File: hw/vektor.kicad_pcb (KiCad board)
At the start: 6 copper layers, 100 x 44 mm, 259 parts, among them J1 Header_2.54mm_10p, J2 0430450818, M1 MHNP_2.5mm, M2 MHNP_2.5mm, M3 MHNP_2.5mm, M4 MHNP_2.5mm, M5 MHNP_2.5mm, Q1 PHPT61002PYCLHX, Q2 PUMH13, Q3 PUMD13, U1 TAS2770, U10 74LVCH1T45GW, U11 74LVCH1T45GW, U12 74LVCH1T45GW, U13 74LVCH1T45GW, U14 74LVCH1T45GW, U15 74LVCH1T45GW, U16 LMZ10501SILR, U17 LMZ10501SILR, U2 TAS2770, U3 TAS2770, U4 ADAU1467, U5 TORX1355(V,F), U6 TOTX1350(V,F), U7 25AA1024, U8 LP3470IM5X-3.08_NOPB, U9 XCL226A0K1H2, X1 NX3225SA-12.288M-STD-CRS-2

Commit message: ...
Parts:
- U5, U6: footprint TOSLINK_VERTICAL -> footprints:TOSLINK_VERTICAL
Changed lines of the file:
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@@
-(kicad_pcb (version 20171130) (host pcbnew "(5.1.0-0)")
+(kicad_pcb (version 20171130) (host pcbnew "(5.1.2-1)-1")
   (general
     (thickness 1.6)
@@
     (add_net P5V0)
   )
+  (module footprints:TOSLINK_VERTICAL (layer B.Cu)
+    (at 141 85 90)
+    (fp_text reference U5 (at 0 -1.905 90) (layer B.SilkS)
+      (effects (font (size 0.8 0.8) (thickness 0.127)) (justify mirror))
+    )
+    (fp_text value "TORX1355(V,F)" (at 0 -6.35 90) (layer B.Fab)
+      (effects (font (size 1 1) (thickness 0.15)) (justify mirror))
+    )
+    (fp_text user TOSLINK (at 0 4.445 90) (layer B.SilkS)
+      (effects (font (size 1 1) (thickness 0.15)) (justify mirror))
+    )
+    (fp_circle (center 0 0.635) (end 0 1.905) (layer B.SilkS) (width 0.15))
+    (fp_line (start 2.54 -2.54) (end -2.54 -2.54) (layer B.SilkS) (width 0.15))
+    (fp_line (start 3.81 -1.27) (end 2.54 -2.54) (layer B.SilkS) (width 0.15))
+    (fp_line (start 3.81 3.81) (end 3.81 -1.27) (layer B.SilkS) (width 0.15))
+    (fp_line (start -3.81 3.81) (end 3.81 3.81) (layer B.SilkS) (width 0.15))
+    (fp_line (start -3.81 -1.27) (end -3.81 3.81) (layer B.SilkS) (width 0.15))
+    (fp_line (start -2.54 -2.54) (end -3.81 -1.27) (layer B.SilkS) (width 0.15))
+    (fp_line (start -7.7 5.25) (end -7.7 -5.25) (layer B.SilkS) (width 0.15))
+    (fp_line (start 7.7 5.25) (end 7.7 -5.25) (layer B.SilkS) (width 0.15))
+    (fp_line (start -7.7 -5.25) (end 7.7 -5.25) (layer B.SilkS) (width 0.15))
+    (fp_line (start -7.7 5.25) (end 7.7 5.25) (layer B.SilkS) (width 0.15))
+    (pad 5 thru_hole circle (at 6.525 0 90) (size 1.524 1.524) (drill 0.762) (layers *.Cu *.Mask)
+      (net 41 "Net-(U5-Pad5)"))
+    (pad 4 thru_hole circle (at -6.525 0 90) (size 1.524 1.524) (drill 0.762) (layers *.Cu *.Mask)
+      (net 40 "Net-(U5-Pad4)"))
+    (pad 3 thru_hole circle (at -2.54 -3.85 90) (size 1.524 1.524) (drill 0.762) (layers *.Cu *.Mask)
+      (net 113 P5V0))
+    (pad 2 thru_hole circle (at 0 -3.85 90) (size 1.524 1.524) (drill 0.762) (layers *.Cu *.Mask)
+      (net 1 GND))
+    (pad 1 thru_hole circle (at 2.54 -3.85 90) (size 1.524 1.524) (drill 0.762) (layers *.Cu *.Mask)
+      (net 132 "Net-(TP57-Pad1)"))
+    (model toslink.step
+      (at (xyz 0 0 0))
+      (scale (xyz 1 1 1))
+      (rotate (xyz 0 0 0))
+    )
+  )
+  (module footprints:TOSLINK_VERTICAL (layer B.Cu)
+    (at 141 111 90)
+    (fp_text reference U6 (at 0 -1.905 90) (layer B.SilkS)
+      (effects (font (size 0.8 0.8) (thickness 0.127)) (justify mirror))
+    )
+    (fp_text value "TOTX1350(V,F)" (at 0 -6.35 90) (layer B.Fab)
+      (effects (font (size 1 1) (thickness 0.15)) (justify mirror))
+    )
+    (fp_text user TOSLINK (at 0 4.445 90) (layer B.SilkS)
+      (effects (font (size 1 1) (thickness 0.15)) (justify mirror))
+    )
+    (fp_circle (center 0 0.635) (end 0 1.905) (layer B.SilkS) (width 0.15))
+    (fp_line (start 2.54 -2.54) (end -2.54 -2.54) (layer B.SilkS) (width 0.15))
+    (fp_line (start 3.81 -1.27) (end 2.54 -2.54) (layer B.SilkS) (width 0.15))
+    (fp_line (start 3.81 3.81) (end 3.81 -1.27) (layer B.SilkS) (width 0.15))
+    (fp_line (start -3.81 3.81) (end 3.81 3.81) (layer B.SilkS) (width 0.15))
+    (fp_line (start -3.81 -1.27) (end -3.81 3.81) (layer B.SilkS) (width 0.15))
+    (fp_line (start -2.54 -2.54) (end -3.81 -1.27) (layer B.SilkS) (width 0.15))
+    (fp_line (start -7.7 5.25) (end -7.7 -5.25) (layer B.SilkS) (width 0.15))
+    (fp_line (start 7.7 5.25) (end 7.7 -5.25) (layer B.SilkS) (width 0.15))
+    (fp_line (start -7.7 -5.25) (end 7.7 -5.25) (layer B.SilkS) (width 0.15))
+    (fp_line (start -7.7 5.25) (end 7.7 5.25) (layer B.SilkS) (width 0.15))
+    (pad 5 thru_hole circle (at 6.525 0 90) (size 1.524 1.524) (drill 0.762) (layers *.Cu *.Mask)
+      (net 42 "Net-(U6-Pad5)"))
+    (pad 4 thru_hole circle (at -6.525 0 90) (size 1.524 1.524) (drill 0.762) (layers *.Cu *.Mask)
+      (net 43 "Net-(U6-Pad4)"))
+    (pad 3 thru_hole circle (at -2.54 -3.85 90) (size 1.524 1.524) (drill 0.762) (layers *.Cu *.Mask)
+      (net 128 "Net-(R19-Pad2)"))
+    (pad 2 thru_hole circle (at 0 -3.85 90) (size 1.524 1.524) (drill 0.762) (layers *.Cu *.Mask)
+      (net 1 GND))
+    (pad 1 thru_hole circle (at 2.54 -3.85 90) (size 1.524 1.524) (drill 0.762) (layers *.Cu *.Mask)
+      (net 44 "Net-(U6-Pad1)"))
+    (model toslink.step
+      (at (xyz 0 0 0))
+      (scale (xyz 1 1 1))
+      (rotate (xyz 0 0 0))
+    )
+  )
   (module footprints:TP_1mm (layer F.Cu)
     (at 202.3 92.3)
@@
     )
   )
-  (module TOSLINK_VERTICAL (layer B.Cu)
-    (at 141 85 90)
-    (fp_text reference U5 (at 0 -1.905 90) (layer B.SilkS)
-      (effects (font (size 0.8 0.8) (thickness 0.127)) (justify mirror))
-    )
-    (fp_text value "TORX1355(V,F)" (at 0 -6.35 90) (layer B.Fab)
-      (effects (font (size 1 1) (thickness 0.15)) (justify mirror))
-    )
-    (fp_line (start -7.7 5.25) (end 7.7 5.25) (layer B.SilkS) (width 0.15))
-    (fp_line (start -7.7 -5.25) (end 7.7 -5.25) (layer B.SilkS) (width 0.15))
-    (fp_line (start 7.7 5.25) (end 7.7 -5.25) (layer B.SilkS) (width 0.15))
-    (fp_line (start -7.7 5.25) (end -7.7 -5.25) (layer B.SilkS) (width 0.15))
-    (fp_line (start -2.54 -2.54) (end -3.81 -1.27) (layer B.SilkS) (width 0.15))
-    (fp_line (start -3.81 -1.27) (end -3.81 3.81) (layer B.SilkS) (width 0.15))
-    (fp_line (start -3.81 3.81) (end 3.81 3.81) (layer B.SilkS) (width 0.15))
-    (fp_line (start 3.81 3.81) (end 3.81 -1.27) (layer B.SilkS) (width 0.15))
-    (fp_line (start 3.81 -1.27) (end 2.54 -2.54) (layer B.SilkS) (width 0.15))
-    (fp_line (start 2.54 -2.54) (end -2.54 -2.54) (layer B.SilkS) (width 0.15))
-    (fp_circle (center 0 0.635) (end 0 1.905) (layer B.SilkS) (width 0.15))
-    (fp_text user TOSLINK (at 0 4.445 90) (layer B.SilkS)
-      (effects (font (size 1 1) (thickness 0.15)) (justify mirror))
-    )
-    (pad 1 thru_hole circle (at 2.54 -3.85 90) (size 1.524 1.524) (drill 0.762) (layers *.Cu *.Mask)
-      (net 132 "Net-(TP57-Pad1)"))
-    (pad 2 thru_hole circle (at 0 -3.85 90) (size 1.524 1.524) (drill 0.762) (layers *.Cu *.Mask)
-      (net 1 GND))
-    (pad 3 thru_hole circle (at -2.54 -3.85 90) (size 1.524 1.524) (drill 0.762) (layers *.Cu *.Mask)
-      (net 113 P5V0))
-    (pad 4 thru_hole circle (at -6.525 0 90) (size 1.524 1.524) (drill 0.762) (layers *.Cu *.Mask)
-      (net 40 "Net-(U5-Pad4)"))
-    (pad 5 thru_hole circle (at 6.525 0 90) (size 1.524 1.524) (drill 0.762) (layers *.Cu *.Mask)
-      (net 41 "Net-(U5-Pad5)"))
-  )
-  (module TOSLINK_VERTICAL (layer B.Cu)
-    (at 141 111 90)
-    (fp_text reference U6 (at 0 -1.905 90) (layer B.SilkS)
-      (effects (font (size 0.8 0.8) (thickness 0.127)) (justify mirror))
-    )
-    (fp_text value "TOTX1350(V,F)" (at 0 -6.35 90) (layer B.Fab)
-      (effects (font (size 1 1) (thickness 0.15)) (justify mirror))
-    )
-    (fp_text user TOSLINK (at 0 4.445 90) (layer B.SilkS)
-      (effects (font (size 1 1) (thickness 0.15)) (justify mirror))
-    )
-    (fp_circle (center 0 0.635) (end 0 1.905) (layer B.SilkS) (width 0.15))
-    (fp_line (start 2.54 -2.54) (end -2.54 -2.54) (layer B.SilkS) (width 0.15))
-    (fp_line (start 3.81 -1.27) (end 2.54 -2.54) (layer B.SilkS) (width 0.15))
-    (fp_line (start 3.81 3.81) (end 3.81 -1.27) (layer B.SilkS) (width 0.15))
-    (fp_line (start -3.81 3.81) (end 3.81 3.81) (layer B.SilkS) (width 0.15))
-    (fp_line (start -3.81 -1.27) (end -3.81 3.81) (layer B.SilkS) (width 0.15))
-    (fp_line (start -2.54 -2.54) (end -3.81 -1.27) (layer B.SilkS) (width 0.15))
-    (fp_line (start -7.7 5.25) (end -7.7 -5.25) (layer B.SilkS) (width 0.15))
-    (fp_line (start 7.7 5.25) (end 7.7 -5.25) (layer B.SilkS) (width 0.15))
-    (fp_line (start -7.7 -5.25) (end 7.7 -5.25) (layer B.SilkS) (width 0.15))
-    (fp_line (start -7.7 5.25) (end 7.7 5.25) (layer B.SilkS) (width 0.15))
-    (pad 5 thru_hole circle (at 6.525 0 90) (size 1.524 1.524) (drill 0.762) (layers *.Cu *.Mask)
-      (net 42 "Net-(U6-Pad5)"))
-    (pad 4 thru_hole circle (at -6.525 0 90) (size 1.524 1.524) (drill 0.762) (layers *.Cu *.Mask)
-      (net 43 "Net-(U6-Pad4)"))
-    (pad 3 thru_hole circle (at -2.54 -3.85 90) (size 1.524 1.524) (drill 0.762) (layers *.Cu *.Mask)
-      (net 128 "Net-(R19-Pad2)"))
-    (pad 2 thru_hole circle (at 0 -3.85 90) (size 1.524 1.524) (drill 0.762) (layers *.Cu *.Mask)
-      (net 1 GND))
-    (pad 1 thru_hole circle (at 2.54 -3.85 90) (size 1.524 1.524) (drill 0.762) (layers *.Cu *.Mask)
-      (net 44 "Net-(U6-Pad1)"))
-  )
   (module RJQ0026A (layer F.Cu)

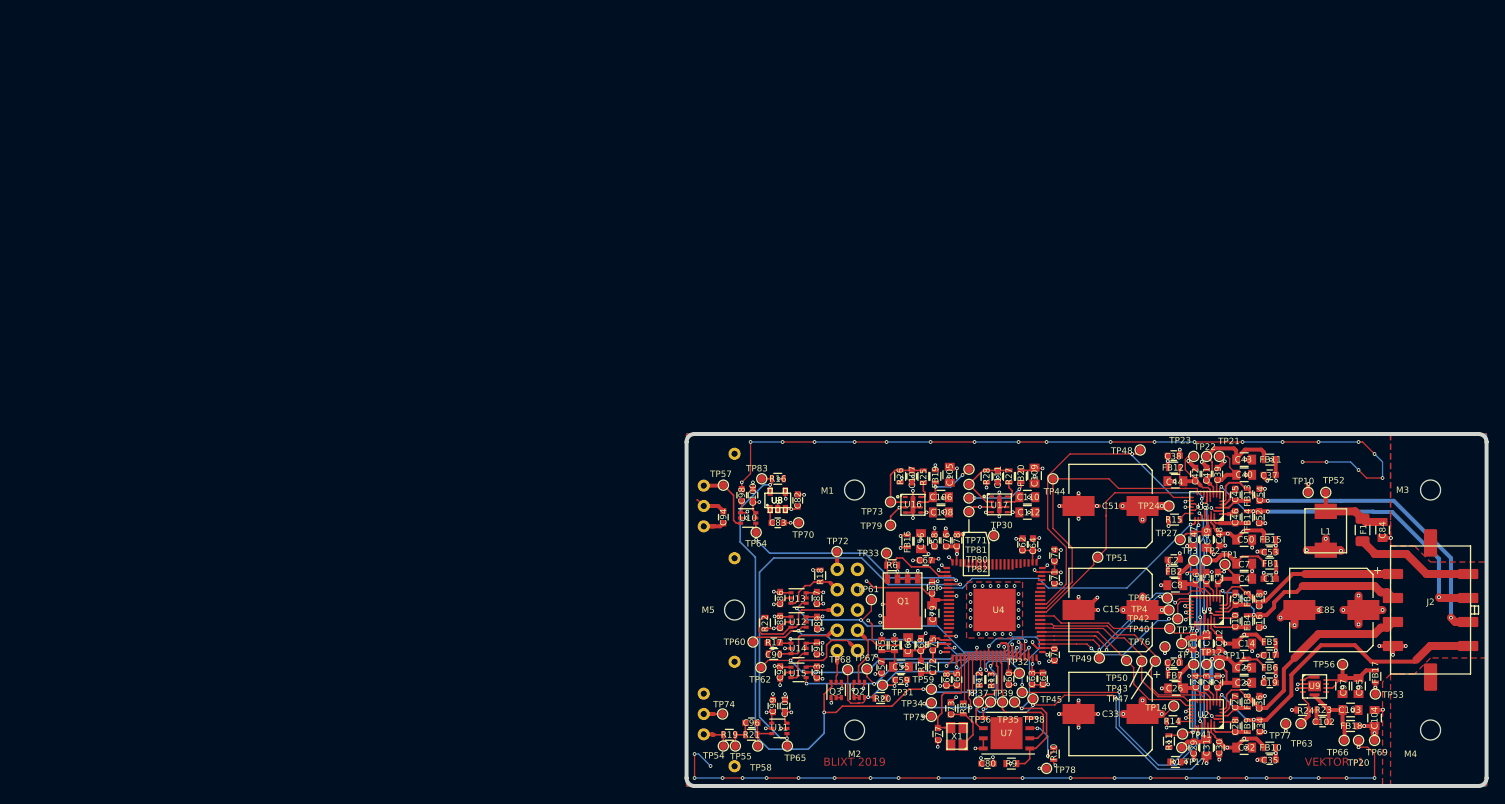
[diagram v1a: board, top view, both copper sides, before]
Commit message: preparing r2
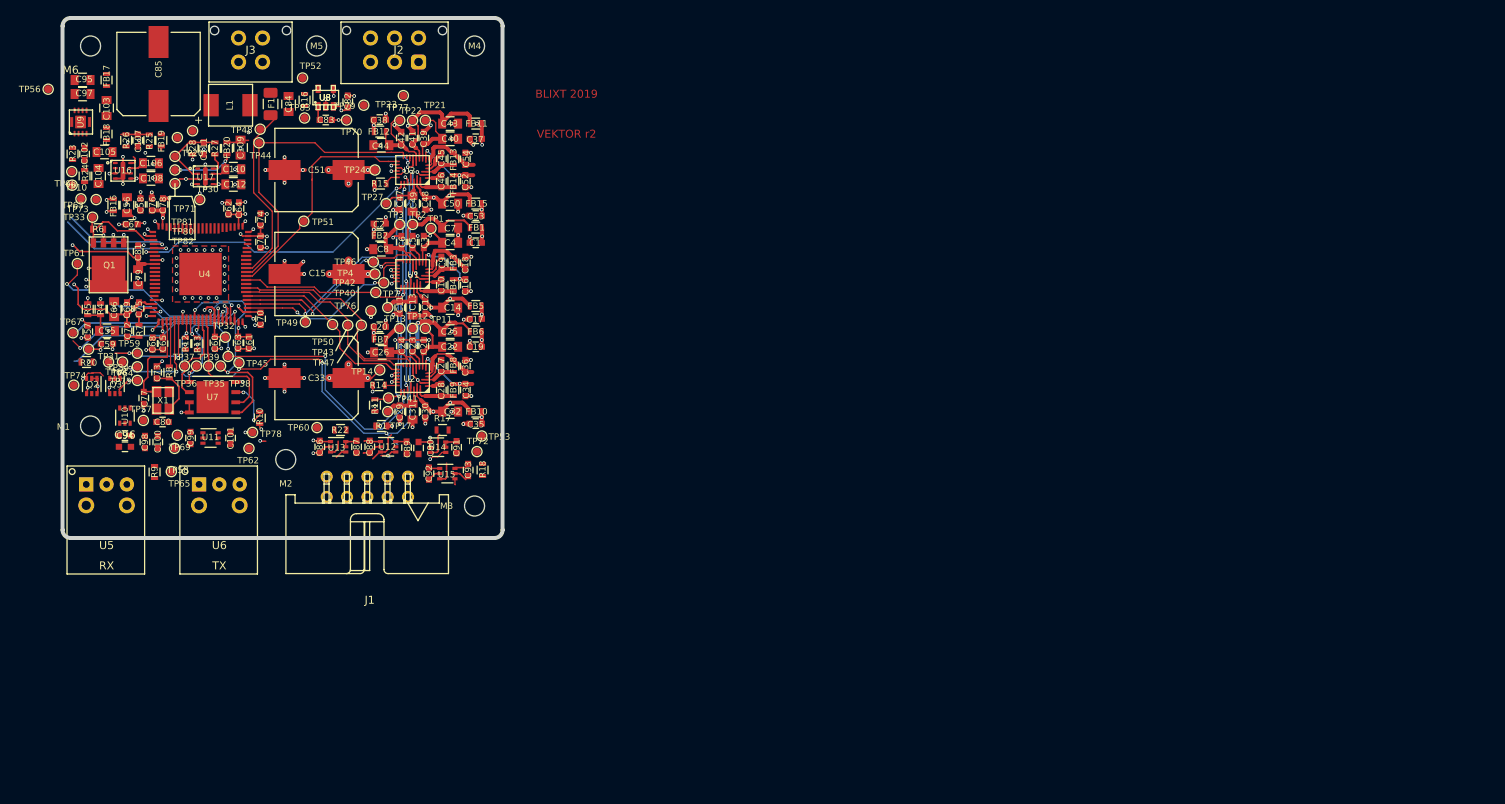
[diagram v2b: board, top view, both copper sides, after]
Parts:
- removed R19: R0603_120R, R0603
- removed R21: R0603_390R, R0603
- removed TP54, TP55: TP, footprints:TP_1mm
- added J3: 430450427, Molex_430450427, F.Cu at (80.5, 28.0)
- added M6: MHNP_2.5mm, footprints:MH_2.5mm, F.Cu at (60.5, 27.5)
- C102: value C0603_18p_50Vdc_C0G_2 -> C0603_18p_100Vdc_C0G
- C107, C111: value C0603_470p_50Vdc_C0G_2 -> C0603_470p_100Vdc_C0G
- C16, C18, C34, C36, C52, C54: value C0603_1n1_50Vdc_X7R -> C0603_1n2_50Vdc_C0G
- C84, C95: value C0805_10u_25Vdc_X7R -> C0805_10u_25Vdc_X7R(Murata)
- C96: value C0603_47p_50Vdc_C0G_2 -> C0603_1u_16Vdc_X7R
- J1: value Header_2.54mm_10p -> TE_5103310-1; footprint footprints:61201021621 -> footprints:TE_5103310_1; moved to F.Cu
- J2: value 0430450818 -> 430450629; footprint Molex_0430450818 -> Molex_430450629
- U5: value TORX1355(V,F) -> PLR135_T10; footprint footprints:TOSLINK_VERTICAL -> PLR135_T10; moved to F.Cu
- U6: value TOTX1350(V,F) -> PLT133_T10W; footprint footprints:TOSLINK_VERTICAL -> PLT133_T10W; moved to F.Cu
- moved TP56 177.1 mm to (55.2, 32.9)
- moved C95 176.6 mm to (59.5, 31.8), turned to 0 degrees
- moved FB17 175.2 mm to (62.5, 31.8)
- moved TP66 174.2 mm to (58.1, 43.2)
- moved C97 174.0 mm to (59.5, 33.5), turned to 0 degrees
- moved C104 173.3 mm to (61.5, 43.8)
- moved C103 172.8 mm to (62.5, 35.2), turned to 90 degrees
- moved FB18 172.2 mm to (62.5, 38.5), turned to 270 degrees
- moved R23 171.0 mm to (58.2, 41.0), turned to 270 degrees
- moved C102 170.3 mm to (59.8, 41.0), turned to 270 degrees
- moved U9 169.6 mm to (59.2, 37.0), turned to 90 degrees
- moved TP63 167.7 mm to (58.2, 44.9)
- moved R24 166.2 mm to (59.8, 43.8), turned to 270 degrees
- moved TP20 164.5 mm to (73.2, 38.1)
- moved C85 161.2 mm to (69.0, 31.0), turned to 90 degrees
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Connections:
- C96 pad 1: Net-(C96-Pad1) -> P5V0
- C96 pad 2: Net-(C96-Pad2) -> GND
- F1 pad 1: /VIN -> Net-(F1-Pad1)
- F1 pad 2: Net-(F1-Pad2) -> /VIN
- J2 pad 1: GND -> /Amplifier 3/AMP_OUT_P_FLT
- J2 pad 5: /Amplifier 2/AMP_OUT_N_FLT -> /Amplifier 3/AMP_OUT_N_FLT
- J2 pad 6: /Amplifier 3/AMP_OUT_P_FLT -> /Amplifier 2/AMP_OUT_N_FLT
- TP58 pad 1: Net-(C96-Pad1) -> Net-(TP58-Pad1)
- U10 pad 5: P1V8 -> P5V0
- U11 pad 3: Net-(C96-Pad1) -> Net-(TP58-Pad1)
- U12 pad 5: P1V8 -> GND
- U13 pad 5: P1V8 -> P3V3
- U14 pad 5: P1V8 -> P3V3
- U15 pad 5: GND -> P3V3
- U5 pad 1: Net-(TP57-Pad1) -> P5V0
- U5 pad 3: P5V0 -> Net-(TP57-Pad1)
- U6 pad 1: Net-(U6-Pad1) -> Net-(TP58-Pad1)
- U6 pad 2: GND -> P5V0
- U6 pad 3: Net-(R19-Pad2) -> GND
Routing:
- net GND: track 399.4 -> 155.8 mm, vias 227 -> 148
- net /RESET_N: track 79.6 -> 15.7 mm, vias 4 -> 2
- net /SPDIF_OUT_1V8: track 52.9 -> 15.2 mm, vias 2 -> 1
- net /Amplifier 3/AMP_OUT_P_FLT: track 44.3 -> 10.4 mm, vias 2 -> 0
- net /Amplifier 3/AMP_OUT_N_FLT: track 41.2 -> 8.83 mm, vias 4 -> 2
- net /Amplifier 2/AMP_OUT_N_FLT: track 41.0 -> 8.73 mm
- net P5V0: track 29.1 -> 3.60 mm, vias 7 -> 1
- net /Amplifier 2/AMP_OUT_P_FLT: track 30.3 -> 9.56 mm
- net /IUSB_MISO: track 37.7 -> 18.2 mm
- net /Amplifier 1/AMP_OUT_N_FLT: track 27.5 -> 8.34 mm
- net /Amplifier 1/AMP_OUT_P_FLT: track 27.0 -> 8.42 mm
- net /SPDIF_IN_1V8: track 30.3 -> 13.9 mm, vias 2 -> 1
- net /DSP/SDATA_OUT2: track 43.8 -> 28.1 mm, vias 2 -> 1
- net P12V: track 20.2 -> 4.50 mm, vias 11 -> 3
- net Net-(F1-Pad2): track 15.0 -> 0.00 mm
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- removed copper zone on B.Cu, net GND
- removed copper zone on In1.Cu, net GND
- removed copper zone on In3.Cu, net GND
- removed copper zone on In4.Cu, net GND
- removed copper zone on F.Cu, net Net-(J2-Pad10)
- removed copper zone on F.Cu, net Net-(J2-Pad9)
- removed copper zone on In3.Cu, net P12V
- removed copper zone on In2.Cu, net P1V8
- removed copper zone on In3.Cu, net P3V3
- removed copper zone on In3.Cu, net P5V0
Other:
- board size 100 x 44 mm -> 55 x 65 mm
- board text added: "VEKTOR r2"
- board text removed: "VEKTOR r1"
